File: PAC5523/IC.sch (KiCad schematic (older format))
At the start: 17 parts, among them U2 ACT4088, U3 MAX3051, U4 AM26LS32, U5 NL17SZ125, U6 RS485, U7 USBLC6-4, U8 USBLC6-4, U9 USBLC6-4

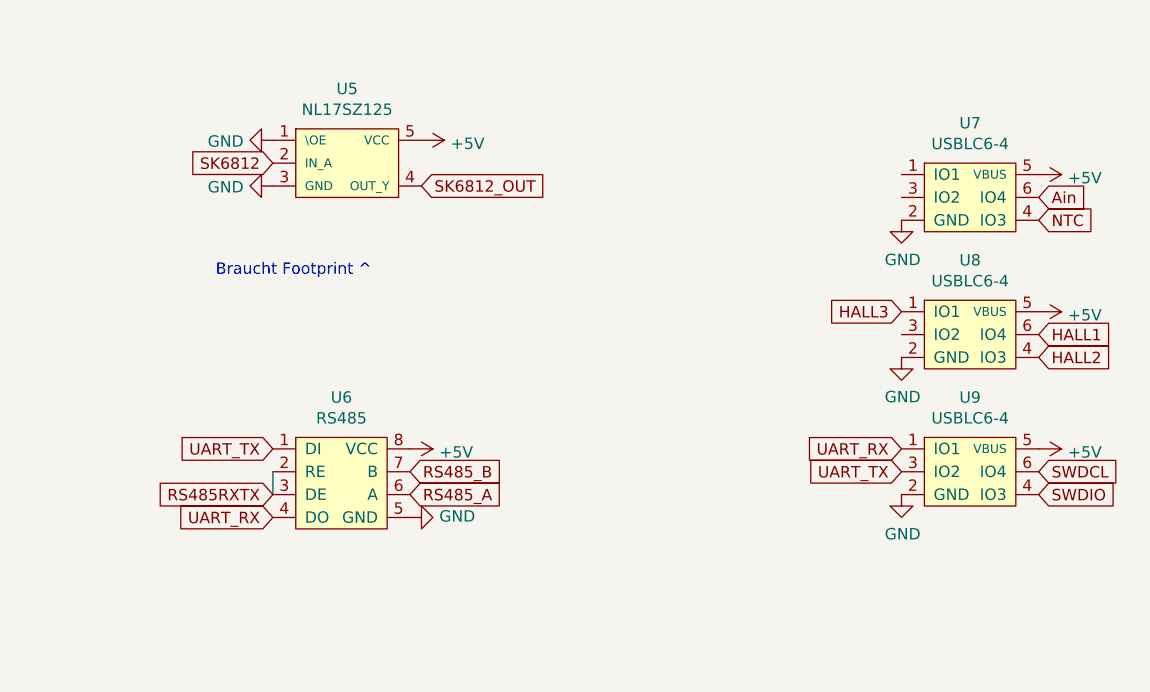
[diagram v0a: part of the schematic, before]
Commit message: wip
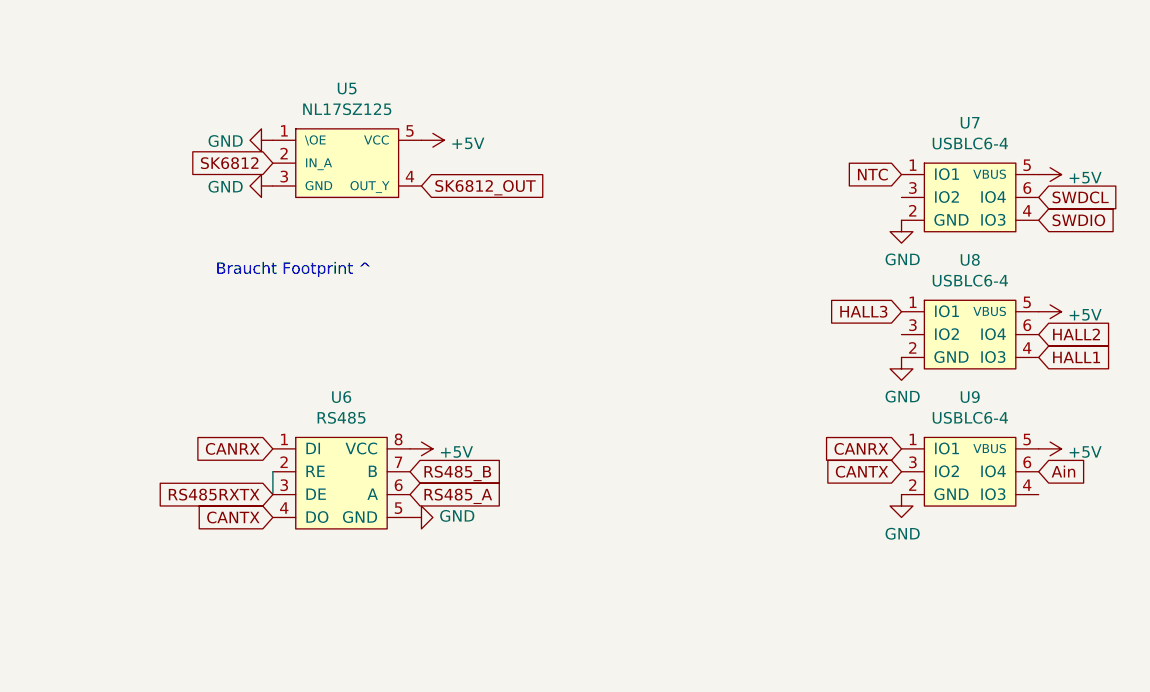
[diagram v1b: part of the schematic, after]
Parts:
- D17: footprint Diode_SMD:D_SMA -> Diode_SMD:D_SOD-123F
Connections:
- net Ain: now also U9.6 (IO4); no longer U7.6 (IO4)
- net CANRX: now also U6.1 (DI), U9.1 (IO1)
- net CANTX: now also U6.4 (DO), U9.3 (IO2)
- net HALL1: now also U8.4 (IO3); no longer U8.6 (IO4)
- net HALL2: now also U8.6 (IO4); no longer U8.4 (IO3)
- net NTC: now also U7.1 (IO1); no longer U7.4 (IO3)
- net SWDCL: now also U7.6 (IO4); no longer U9.6 (IO4)
- net SWDIO: now also U7.4 (IO3); no longer U9.4 (IO3)
- removed net UART_RX: U6.4 (DO), U9.1 (IO1)
- removed net UART_TX: U6.1 (DI), U9.3 (IO2)
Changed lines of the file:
@@
 F 0 "D17" H 2550 2005 50  0000 C CNN
 F 1 "SS310" H 2550 1914 50  0000 C CNN
-F 2 "Diode_SMD:D_SMA" V 2550 1800 50  0001 C CNN
+F 2 "Diode_SMD:D_SOD-123F" V 2550 1800 50  0001 C CNN
 F 3 "~" V 2550 1800 50  0001 C CNN
 	1    2550 1800
@@
 Wire Wire Line
 	6200 4550 6200 4650
-Text GLabel 6200 4750 0    50   Input ~ 0
-UART_RX
-Text GLabel 6200 4450 0    50   Input ~ 0
-UART_TX
 $Comp
 L otter:RS485 U6
@@
 	1    0    0    -1
 $EndComp
+Text GLabel 9550 3350 2    50   Input ~ 0
+SWDCL
+Text GLabel 9550 3450 2    50   Input ~ 0
+SWDIO
+Text GLabel 8950 3250 0    50   Input ~ 0
+NTC
 Text GLabel 9550 4550 2    50   Input ~ 0
-SWDCL
-Text GLabel 9550 4650 2    50   Input ~ 0
-SWDIO
-Text GLabel 9550 3450 2    50   Input ~ 0
-NTC
-Text GLabel 9550 3350 2    50   Input ~ 0
 Ain
 $Comp
@@
 	1    0    0    -1
 $EndComp
-Text GLabel 8950 4450 0    50   Input ~ 0
-UART_RX
-Text GLabel 8950 4550 0    50   Input ~ 0
-UART_TX
 $Comp
 L power:GND #PWR0166
@@
 Text GLabel 8950 3850 0    50   Input ~ 0
 HALL3
+Text GLabel 9550 3950 2    50   Input ~ 0
+HALL2
 Text GLabel 9550 4050 2    50   Input ~ 0
-HALL2
-Text GLabel 9550 3950 2    50   Input ~ 0
 HALL1
 $Comp
@@
 Text GLabel 2350 3600 0    50   Input ~ 0
 CANTX
+Text GLabel 8950 4450 0    50   Input ~ 0
+CANRX
+Text GLabel 8950 4550 0    50   Input ~ 0
+CANTX
+Text GLabel 6200 4750 0    50   Input ~ 0
+CANTX
+Text GLabel 6200 4450 0    50   Input ~ 0
+CANRX
 $EndSCHEMATC

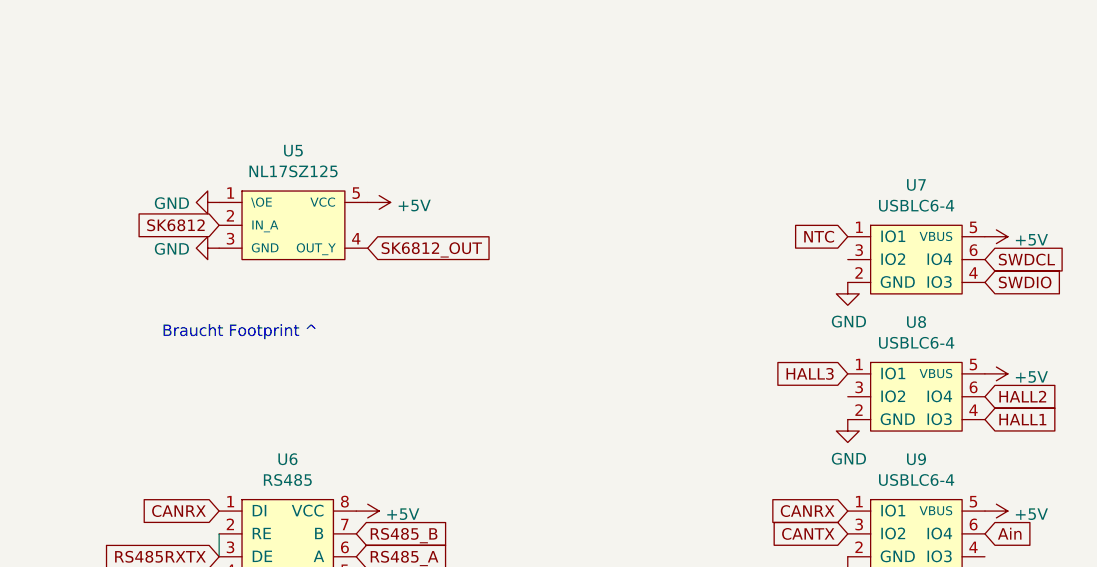
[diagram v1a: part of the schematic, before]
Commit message: wip
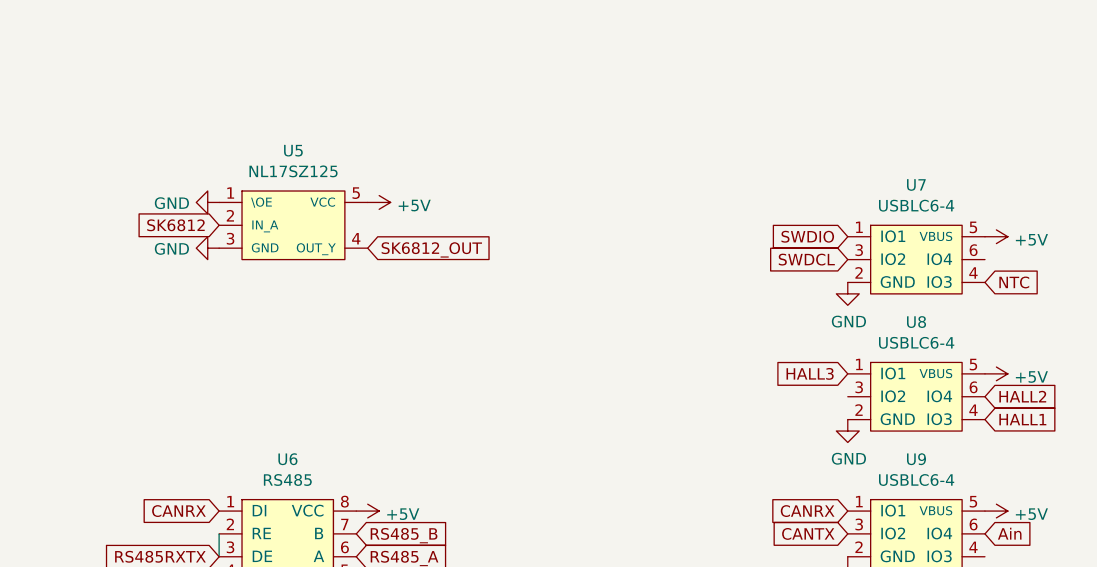
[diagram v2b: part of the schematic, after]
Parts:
- U5: footprint Package_TO_SOT_SMD:SOT-23-5 -> Package_TO_SOT_SMD:SOT-353_SC-70-5
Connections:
- net NTC: now also U7.4 (IO3); no longer U7.1 (IO1)
- net SWDCL: now also U7.3 (IO2); no longer U7.6 (IO4)
- net SWDIO: now also U7.1 (IO1); no longer U7.4 (IO3)
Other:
- note removed: "Braucht Footprint ^"
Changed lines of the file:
@@
 	1    0    0    -1
 $EndComp
-Text Notes 5950 3700 0    50   ~ 0
-Braucht Footprint ^
 Text GLabel 6850 3300 2    50   Input ~ 0
 SK6812_OUT
@@
 F 0 "U5" H 6525 3525 50  0000 C CNN
 F 1 "NL17SZ125" H 6525 3434 50  0000 C CNN
-F 2 "Package_TO_SOT_SMD:SOT-23-5" H 6500 3400 50  0001 C CNN
+F 2 "Package_TO_SOT_SMD:SOT-353_SC-70-5" H 6500 3400 50  0001 C CNN
 F 3 "https://lcsc.com/product-detail/Logic-ICs_ON-Semicon_NL17SZ125DFT2G_ON-Semicon-ON-NL17SZ125DFT2G_C97774.html" H 6500 3400 50  0001 C CNN
 	1    6500 3200
@@
 	1    0    0    -1
 $EndComp
-Text GLabel 9550 3350 2    50   Input ~ 0
+Text GLabel 8950 3350 0    50   Input ~ 0
 SWDCL
+Text GLabel 8950 3250 0    50   Input ~ 0
+SWDIO
 Text GLabel 9550 3450 2    50   Input ~ 0
-SWDIO
-Text GLabel 8950 3250 0    50   Input ~ 0
 NTC
 Text GLabel 9550 4550 2    50   Input ~ 0
